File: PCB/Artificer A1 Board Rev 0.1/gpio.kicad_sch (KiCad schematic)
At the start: 1 part, among them J1 Conn_02x20_Odd_Even

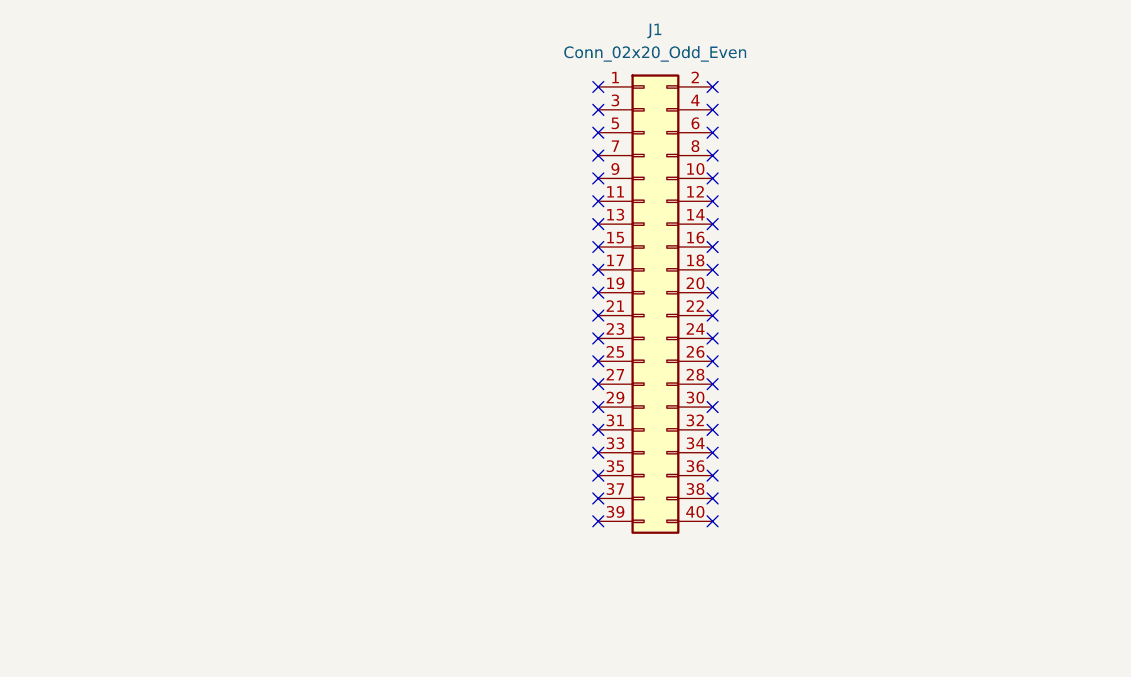
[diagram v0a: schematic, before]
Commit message: more routing and decoupling
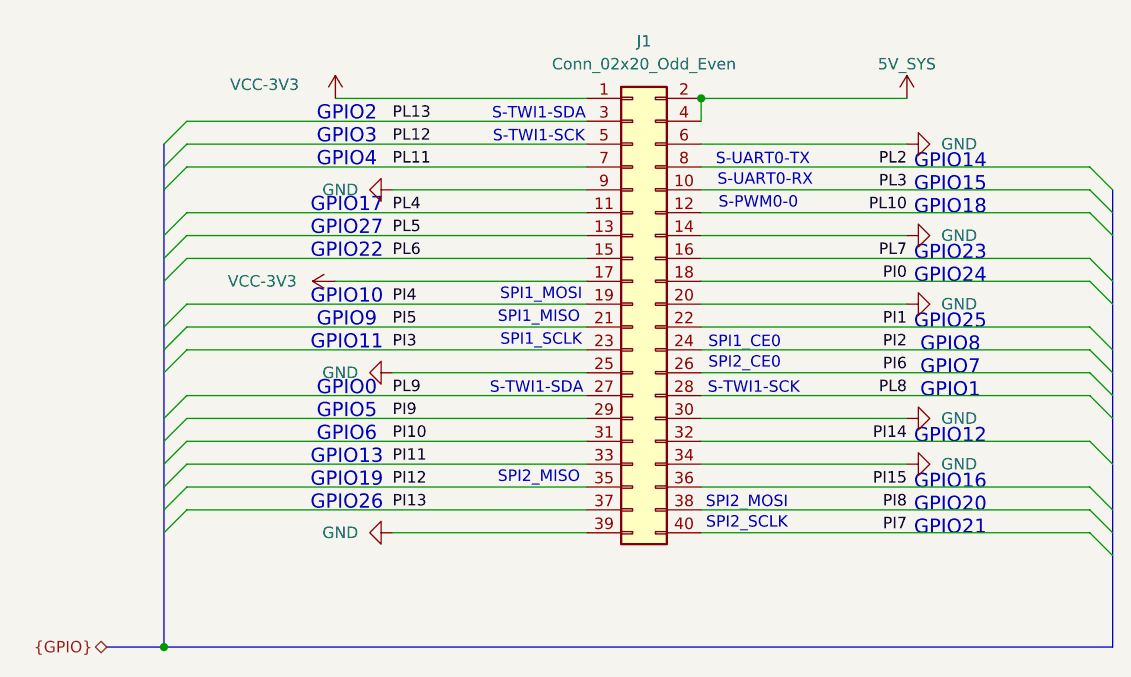
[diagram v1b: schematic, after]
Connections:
- net VCC-3V3: now reaches J1.1 (Pin_1)
- net VCC-3V3: now also J1.17 (Pin_17)
- net PL3: now reaches J1.10 (Pin_10)
- net PL4: now reaches J1.11 (Pin_11)
- net PL10: now reaches J1.12 (Pin_12)
- net PL5: now reaches J1.13 (Pin_13)
- net GND: now reaches J1.14 (Pin_14)
- net GND: now also J1.20 (Pin_20), J1.25 (Pin_25), J1.30 (Pin_30), J1.34 (Pin_34), J1.39 (Pin_39), J1.6 (Pin_6), J1.9 (Pin_9)
- net PL6: now reaches J1.15 (Pin_15)
- net PL7: now reaches J1.16 (Pin_16)
- net PI0: now reaches J1.18 (Pin_18)
- net PI4: now reaches J1.19 (Pin_19)
- net 5V_SYS: now reaches J1.2 (Pin_2)
- net 5V_SYS: now also J1.4 (Pin_4)
- net PI5: now reaches J1.21 (Pin_21)
- net PI1: now reaches J1.22 (Pin_22)
- net PI3: now reaches J1.23 (Pin_23)
- net PI2: now reaches J1.24 (Pin_24)
- net PI6: now reaches J1.26 (Pin_26)
- net PL9: now reaches J1.27 (Pin_27)
- net PL8: now reaches J1.28 (Pin_28)
- net PI9: now reaches J1.29 (Pin_29)
- net PL13: now reaches J1.3 (Pin_3)
- net PI10: now reaches J1.31 (Pin_31)
- net PI14: now reaches J1.32 (Pin_32)
- net PI11: now reaches J1.33 (Pin_33)
- net PI12: now reaches J1.35 (Pin_35)
- net PI15: now reaches J1.36 (Pin_36)
- net PI13: now reaches J1.37 (Pin_37)
- net PI8: now reaches J1.38 (Pin_38)
- net PI7: now reaches J1.40 (Pin_40)
- net PL12: now reaches J1.5 (Pin_5)
- net PL11: now reaches J1.7 (Pin_7)
- net PL2: now reaches J1.8 (Pin_8)
- no-connect marks 40 -> 0
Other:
- note added: "GPIO14 GPIO15 GPIO18 GPIO23 GPIO24 GPIO25 GPIO8 GPIO7 GPIO1 GPIO12 GPIO16 GPIO20 GPIO21"
- note added: "GPIO2 GPIO3 GPIO4 GPIO17 GPIO27 GPIO22 GPIO10 GPIO9 GPIO11 GPIO0 GPIO5 GPIO6 GPIO13 GPIO19 GPIO26"
- note added: "S-PWM0-0"
- note added: "S-TWI1-SCK"
- note added: "S-TWI1-SDA"
- note added: "S-UART0-RX"
- note added: "S-UART0-TX"
- note added: "SPI1_CE0"
- note added: "SPI1_MISO"
- note added: "SPI1_MOSI"
- note added: "SPI1_SCLK"
- note added: "SPI2_CE0"
- note added: "SPI2_MISO"
- note added: "SPI2_MOSI"
- note added: "SPI2_SCLK"
